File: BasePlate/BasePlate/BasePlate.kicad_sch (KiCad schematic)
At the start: 18 parts, among them J1 JST_BM04B-GHS-TBT, J10 XT30UPB-M, J11 XT30UPB-M, J12 XT30UPB-M, J13 XT30UPB-M, J14 XT30UPB-M, J15 JST_B3B-XH-A, J2 1586842-6, J3 JST_BM03B-GHS-TBT, J4 JST_BM04B-GHS-TBT, J5 JST_BM04B-GHS-TBT, J6 JST_BM04B-GHS-TBT, J7 JST_BM04B-GHS-TBT, J8 JST_BM04B-GHS-TBT, J9 XH 2 Pin

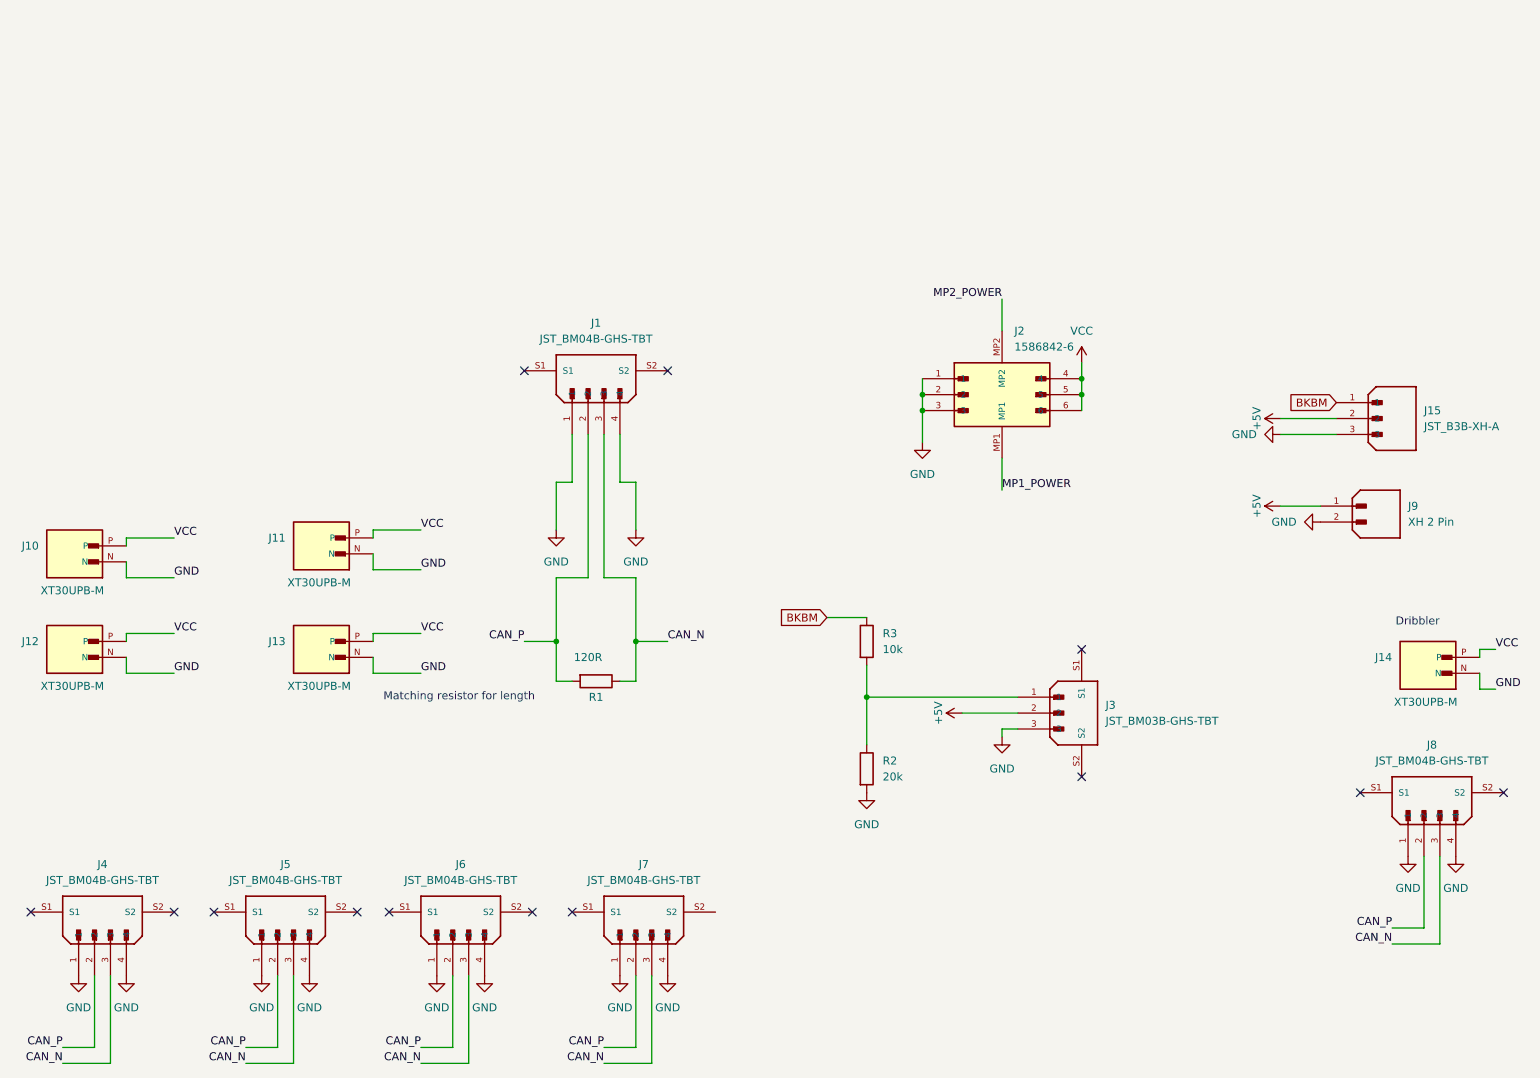
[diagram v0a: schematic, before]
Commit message: update
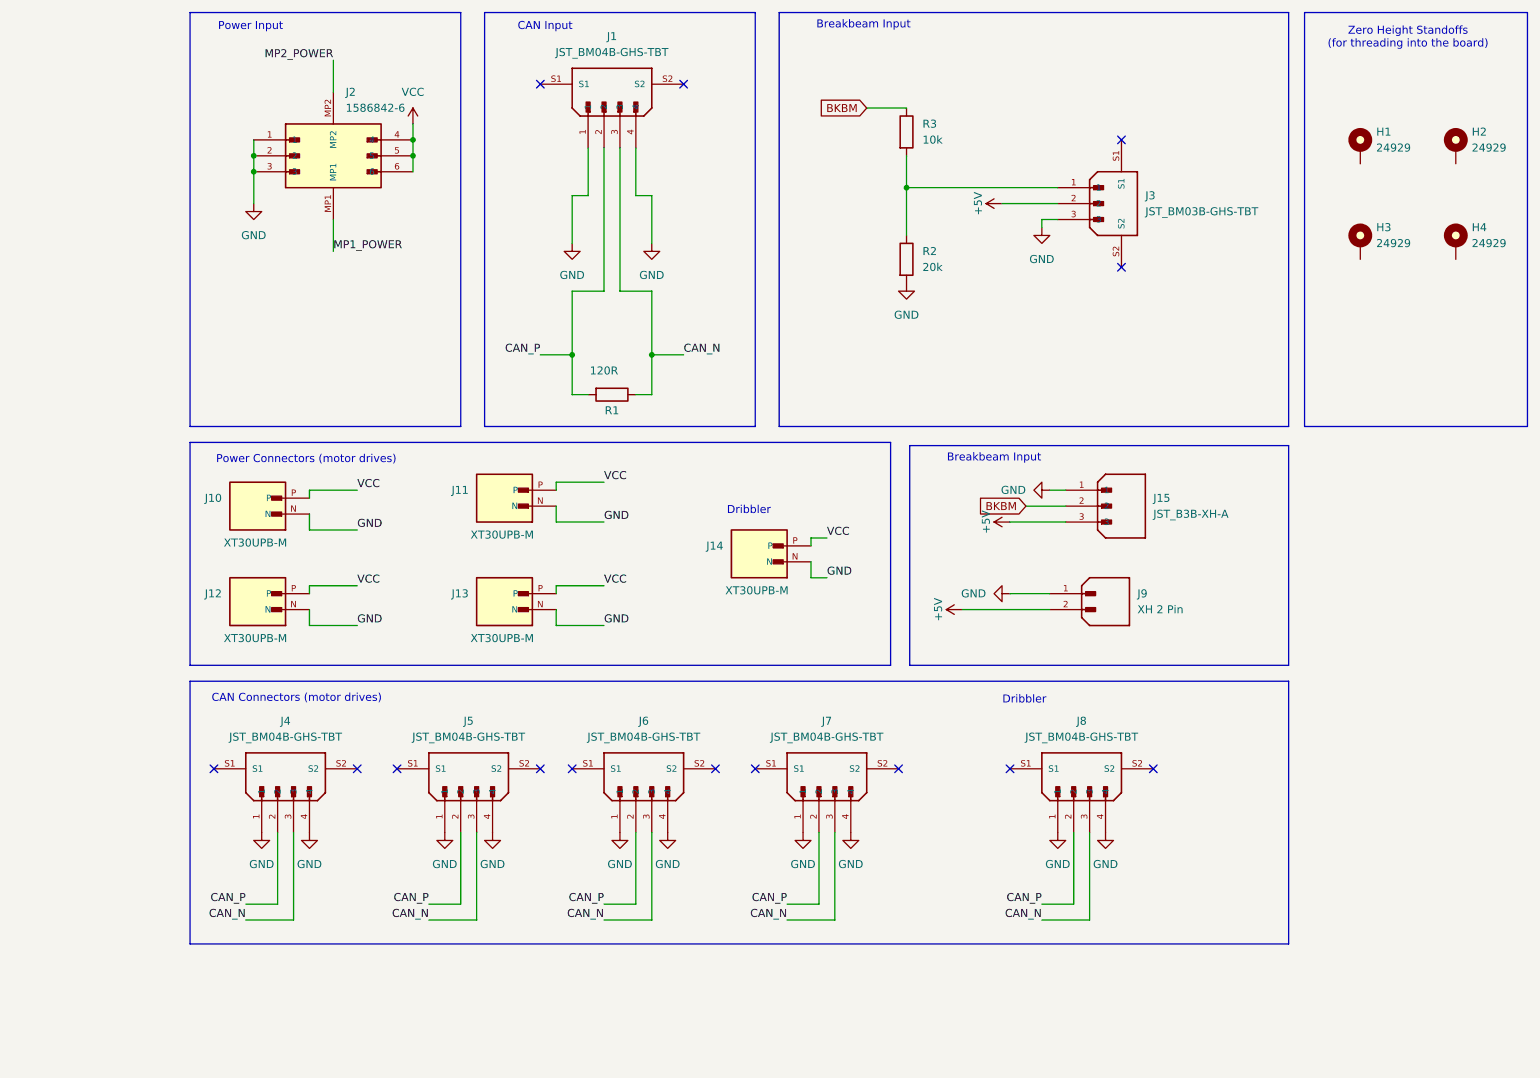
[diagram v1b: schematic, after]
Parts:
- added H1, H2, H3, H4: 24929, bots:Keystone_24929, symbol bots:ZeroH_Keystone24929_Pad
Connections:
- net +5V: now also J15.3, J9.2; no longer J15.2, J9.1
- net BKBM: now also J15.2; no longer J15.1
- net GND: now also J15.1, J9.1; no longer J15.3, J9.2
- no-connect marks 13 -> 14
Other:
- note added: "Breakbeam Input"
- note added: "CAN Connectors (motor drives)"
- note added: "CAN Input"
- note added: "Power Connectors (motor drives)"
- note added: "Power Input"
- note added: "Zero Height Standoffs (for threading into the board)"
- note removed: "Matching resistor for length"
- moved on the sheet: J1, J15, J2, J3, J4, J5, J6, J7, J8, J9, R1, R2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
